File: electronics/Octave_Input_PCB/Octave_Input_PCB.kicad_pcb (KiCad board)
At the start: 2 copper layers, 86.4 x 95.9 mm, 38 parts, among them SW1 SW_Hot_Swap_Socket, SW10 SW_Hot_Swap_Socket, SW11 SW_Hot_Swap_Socket, SW12 SW_Hot_Swap_Socket, SW13 SW_Hot_Swap_Socket, SW14 Alps_Alpine_RKJXV1224, SW15 Bourns_PEC12R-4xxxF-Sxxx, SW2 SW_Hot_Swap_Socket, SW3 SW_Hot_Swap_Socket, SW4 SW_Hot_Swap_Socket, SW5 SW_Hot_Swap_Socket, SW6 SW_Hot_Swap_Socket, SW7 SW_Hot_Swap_Socket, SW8 SW_Hot_Swap_Socket, SW9 SW_Hot_Swap_Socket, U1 Adafruit_QT_Py_RP2040, U2 Raspberry_Pi_RP2040

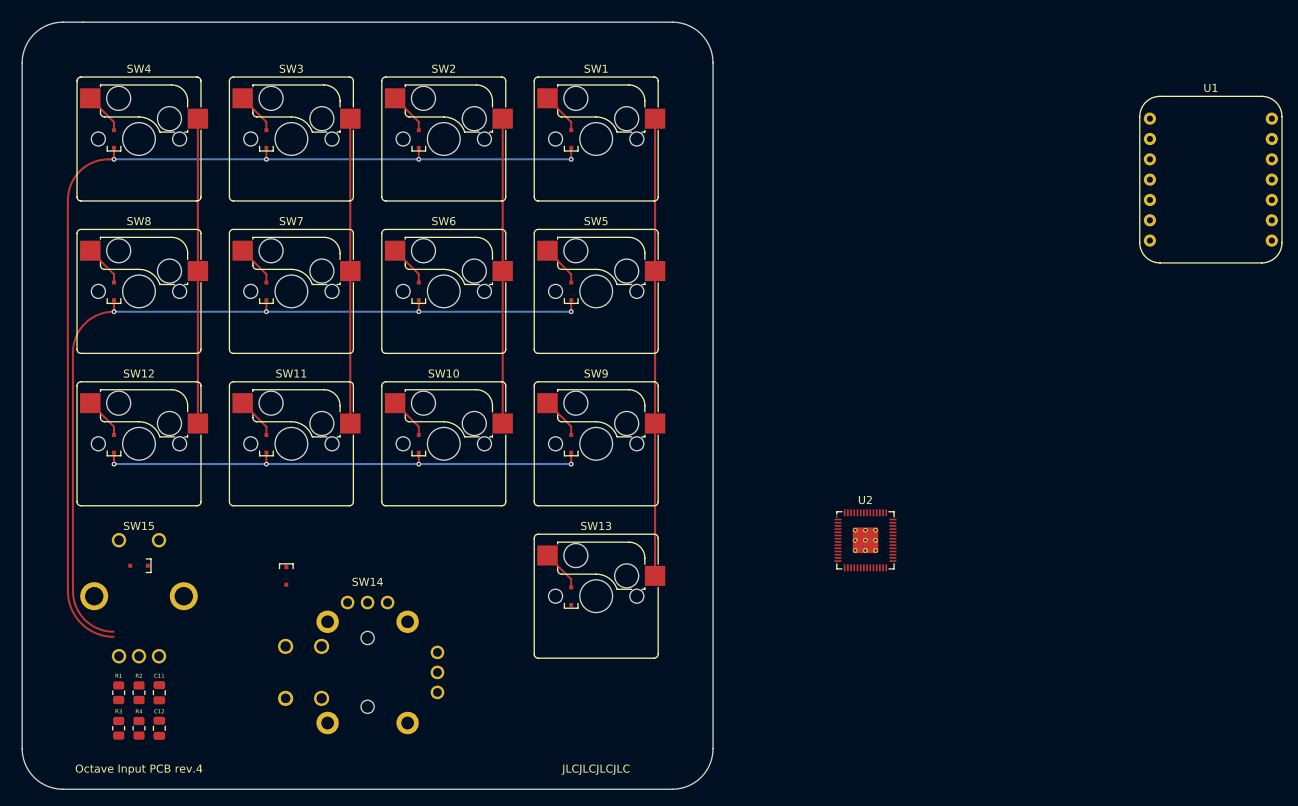
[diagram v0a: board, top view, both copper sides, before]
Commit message: [WIP] Update schematic and PCB
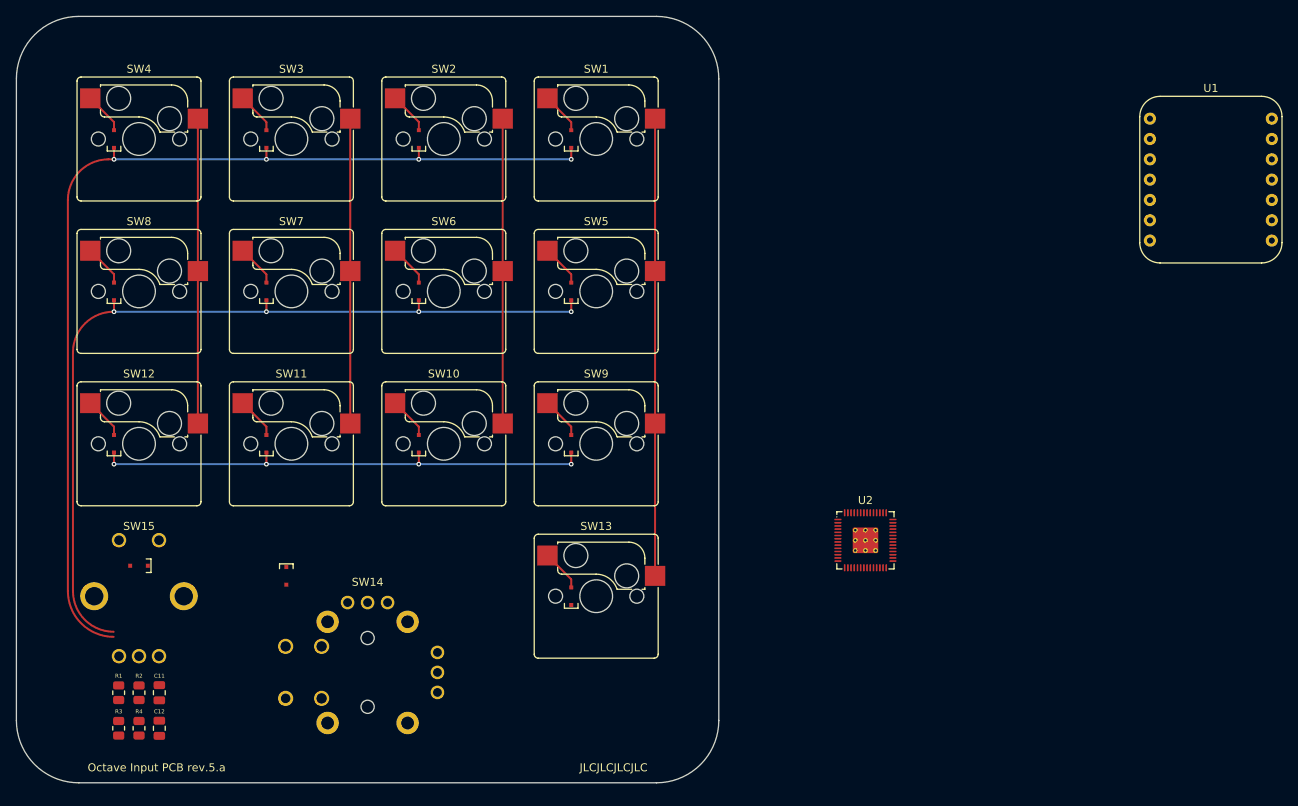
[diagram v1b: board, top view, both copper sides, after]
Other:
- board size 86.4 x 95.9 mm -> 87.8 x 95.8 mm
- board text added: "Octave Input PCB rev.5.a"
- board text removed: "Octave Input PCB rev.4"
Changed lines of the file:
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@@
   (title_block
     (title "Octave - Input PCB")
-    (date "2022-05-05")
+    (date "2022-05-06")
     (rev "5.a")
     (comment 4 "https://github.com/takayoshiotake/octave-12-key-macropad")
@@
     )
   )
-  (gr_line (start 123.825 42.545) (end 50.165 42.545) (layer "Edge.Cuts") (width 0.1))
-  (gr_line (start 47.625 138.43) (end 123.825 138.43) (layer "Edge.Cuts") (width 0.1))
-  (gr_arc (start 47.625 138.43) (mid 44.032898 136.942102) (end 42.545 133.35) (layer "Edge.Cuts") (width 0.1))
-  (gr_line (start 50.165 42.545) (end 47.625 42.545) (layer "Edge.Cuts") (width 0.1))
-  (gr_arc (start 128.905 133.35) (mid 127.417102 136.942102) (end 123.825 138.43) (layer "Edge.Cuts") (width 0.1))
-  (gr_arc (start 42.545 47.625) (mid 44.032898 44.032898) (end 47.625 42.545) (layer "Edge.Cuts") (width 0.1))
-  (gr_arc (start 123.825 42.545) (mid 127.417102 44.032898) (end 128.905 47.625) (layer "Edge.Cuts") (width 0.1))
-  (gr_line (start 128.905 133.35) (end 128.905 47.625) (layer "Edge.Cuts") (width 0.1))
-  (gr_line (start 42.545 47.625) (end 42.545 133.35) (layer "Edge.Cuts") (width 0.1))
-  (gr_rect (start 37.725 37.725) (end 133.725 143.25) (layer "F.Fab") (width 0.12) (fill none))
+  (gr_rect (start 41.825 41.825) (end 129.625 137.625) (layer "Cmts.User") (width 0.15) (fill none))
+  (gr_rect (start 41.825 41.825) (end 49.625 49.625) (layer "Cmts.User") (width 0.15) (fill none))
+  (gr_rect (start 121.825 129.825) (end 129.625 137.625) (layer "Cmts.User") (width 0.15) (fill none))
+  (gr_rect (start 121.825 41.825) (end 129.625 49.625) (layer "Cmts.User") (width 0.15) (fill none))
+  (gr_rect (start 41.825 129.825) (end 49.625 137.625) (layer "Cmts.User") (width 0.15) (fill none))
+  (gr_arc (start 121.825 41.825) (mid 127.340433 44.109567) (end 129.625 49.625) (layer "Edge.Cuts") (width 0.1))
+  (gr_arc (start 129.625 129.825) (mid 127.340433 135.340433) (end 121.825 137.625) (layer "Edge.Cuts") (width 0.1))
+  (gr_arc (start 41.825 49.625) (mid 44.109567 44.109567) (end 49.625 41.825) (layer "Edge.Cuts") (width 0.1))
+  (gr_line (start 121.825 41.825) (end 49.625 41.825) (layer "Edge.Cuts") (width 0.1))
+  (gr_line (start 41.825 49.625) (end 41.825 129.825) (layer "Edge.Cuts") (width 0.1))
+  (gr_line (start 49.625 137.625) (end 121.825 137.625) (layer "Edge.Cuts") (width 0.1))
+  (gr_line (start 129.625 129.825) (end 129.625 49.625) (layer "Edge.Cuts") (width 0.1))
+  (gr_arc (start 49.625 137.625) (mid 44.109567 135.340433) (end 41.825 129.825) (layer "Edge.Cuts") (width 0.1))
   (gr_rect (start 76.2 114.3) (end 95.25 133.35) (layer "F.Fab") (width 0.15) (fill none))
   (gr_rect (start 47.625 104.775) (end 66.675 123.825) (layer "F.Fab") (width 0.15) (fill none))
-  (gr_text "JLCJLCJLCJLC" (at 114.3 135.89) (layer "F.SilkS")
-    (effects (font (size 1 1) (thickness 0.15)))
-  )
-  (gr_text "Octave Input PCB rev.4" (at 57.15 135.89) (layer "F.SilkS")
-    (effects (font (size 1 1) (thickness 0.15)))
+  (gr_text "JLCJLCJLCJLC" (at 120.725 135.725) (layer "F.SilkS")
+    (effects (font (size 1 1) (thickness 0.15)) (justify right))
+  )
+  (gr_text "Octave Input PCB rev.5.a" (at 50.725 135.725) (layer "F.SilkS")
+    (effects (font (size 1 1) (thickness 0.15)) (justify left))
   )
   (dimension (type aligned) (layer "Cmts.User")
-    (pts (xy 42.545 47.625) (xy 128.905 47.625))
-    (height -14.605)
-    (gr_text "3.4000 in" (at 85.725 31.87) (layer "Cmts.User")
-      (effects (font (size 1 1) (thickness 0.15)))
-    )
-    (format (units 0) (units_format 1) (precision 4))
+    (pts (xy 49.625 49.625) (xy 44.109567 44.109567))
+    (height -15.715448)
+    (gr_text "7.8 mm" (at 36.567957 57.166611 -45) (layer "Cmts.User")
+      (effects (font (size 1 1) (thickness 0.15)))
+    )
+    (format (units 3) (units_format 1) (precision 1))
     (style (thickness 0.15) (arrow_length 1.27) (text_position_mode 0) (extension_height 0.58642) (extension_offset 0.5) keep_text_aligned)
   )
   (dimension (type aligned) (layer "Cmts.User")
-    (pts (xy 123.19 42.545) (xy 123.19 138.43))
-    (height -15.24)
-    (gr_text "3.7750 in" (at 137.28 90.4875 90) (layer "Cmts.User")
-      (effects (font (size 1 1) (thickness 0.15)))
-    )
-    (format (units 0) (units_format 1) (precision 4))
+    (pts (xy 129.625 41.825) (xy 129.625 137.625))
+    (height -30.395)
+    (gr_text "95.8 mm" (at 158.87 89.725 90) (layer "Cmts.User")
+      (effects (font (size 1 1) (thickness 0.15)))
+    )
+    (format (units 3) (units_format 1) (precision 1))
     (style (thickness 0.15) (arrow_length 1.27) (text_position_mode 0) (extension_height 0.58642) (extension_offset 0.5) keep_text_aligned)
   )
+  (dimension (type aligned) (layer "Cmts.User")
+    (pts (xy 41.825 41.825) (xy 129.625 41.825))
+    (height -5.63)
+    (gr_text "87.8 mm" (at 85.725 35.045) (layer "Cmts.User")
+      (effects (font (size 1 1) (thickness 0.15)))
+    )
+    (format (units 3) (units_format 1) (precision 1))
+    (style (thickness 0.15) (arrow_length 1.27) (text_position_mode 0) (extension_height 0.58642) (extension_offset 0.5) keep_text_aligned)
+  )
